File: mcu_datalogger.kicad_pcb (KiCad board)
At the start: 2 copper layers, 30.3 x 39.1 mm, 29 parts, among them J1 Conn_01x04_Pin, J2 Conn_01x04_Pin, J3 Conn_01x09_Pin, J4 Conn_02x03_Odd_Even, U1 24LC1025, U2 DS1337S_, U3 24LC1025, U4 ATMEGA328P-AU_SL044, Y1 32.768 KHz, Y2 16 MHz

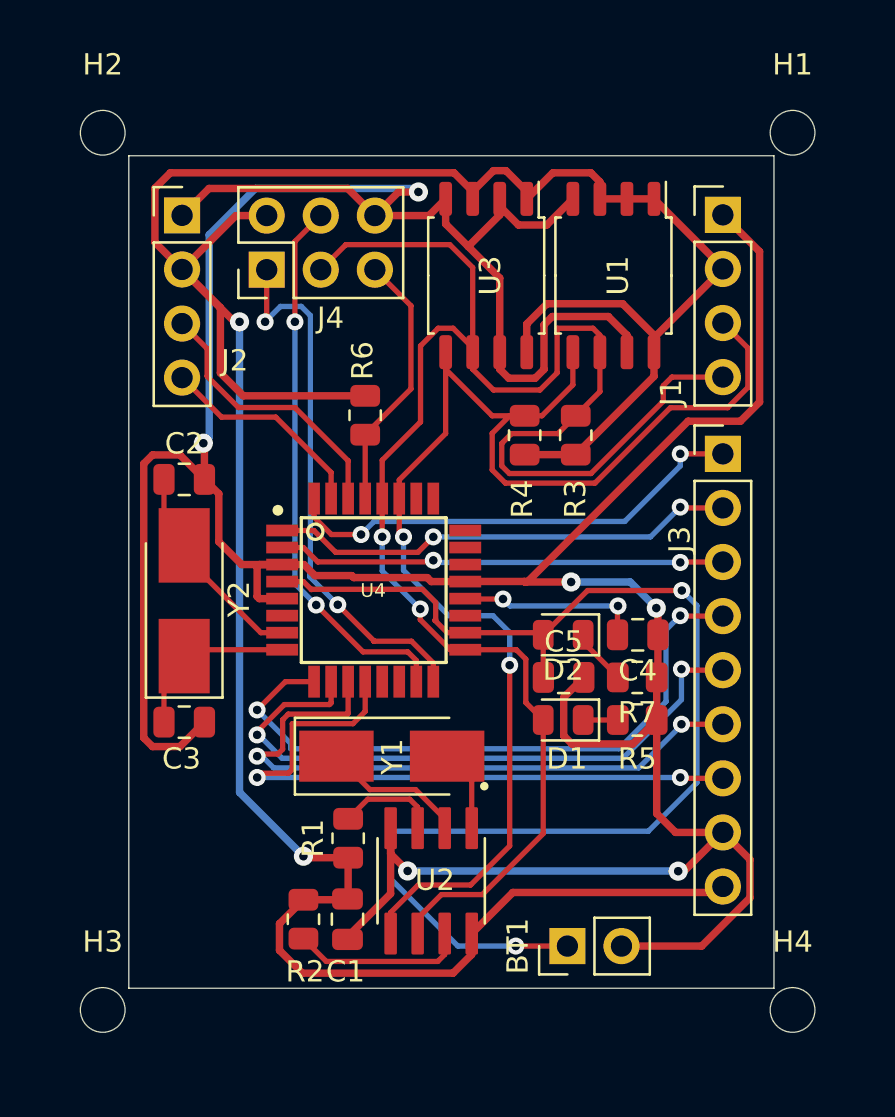
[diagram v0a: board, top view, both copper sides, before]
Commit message: PCB final
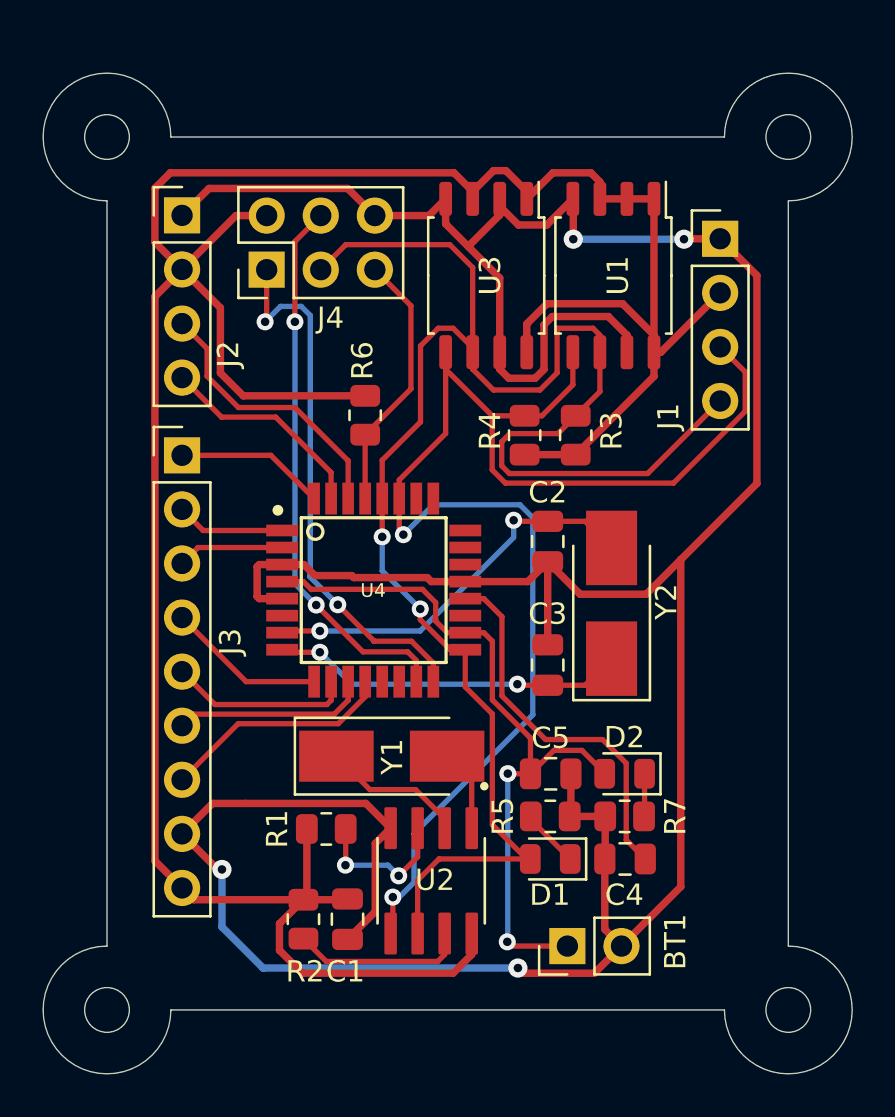
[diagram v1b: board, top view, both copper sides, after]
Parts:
- moved J3 25.4 mm to (146.5, 76.0)
- moved Y2 20.1 mm to (166.7, 82.9)
- moved C2 17.3 mm to (163.7, 80.0), turned to -90 degrees
- moved C3 17.3 mm to (163.7, 85.8), turned to 90 degrees
- moved C4 10.5 mm to (167.3, 94.9), turned to 0 degrees
- moved D2 7.14 mm to (167.3, 90.9)
- moved D1 6.56 mm to (163.8, 94.9)
- moved R7 6.55 mm to (167.3, 92.9), turned to 0 degrees
- moved R5 6.10 mm to (163.8, 92.9)
- moved C5 4.57 mm to (163.8, 90.9)
- moved J1 1.13 mm to (171.8, 65.8)
- moved R1 1.12 mm to (153.3, 93.5), turned to 0 degrees
- moved H1 0.28 mm to (175.0, 61.0)
- moved H2 0.28 mm to (143.0, 61.0)
- moved H3 0.20 mm to (143.0, 102.0)
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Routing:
- net GND: track 194.2 -> 166.9 mm, vias 6 -> 4
- net Net-(BT1-+): track 59.8 -> 34.9 mm
- net /D5: track 30.6 -> 7.45 mm, vias 2 -> 0
- net /D6: track 30.1 -> 8.60 mm, vias 2 -> 0
- net /D7: track 30.4 -> 9.17 mm, vias 2 -> 0
- net /D8: track 30.9 -> 10.9 mm, vias 2 -> 0
- net /D3: track 22.0 -> 5.11 mm, vias 2 -> 0
- net /D4: track 21.1 -> 5.01 mm, vias 2 -> 0
- net /D2: track 22.3 -> 7.04 mm, vias 2 -> 0
- net Net-(U4-AREF): track 8.68 -> 17.8 mm, vias 2 -> 0
- net Net-(U4-PB6): track 10.1 -> 18.7 mm, vias 0 -> 2
- net Net-(U4-PB7): track 8.22 -> 16.7 mm, vias 0 -> 2
- net /Vcc: track 139.6 -> 133.8 mm, vias 2 -> 0
- net Net-(U2-~{INTA}): track 4.79 -> 7.02 mm, vias 0 -> 2
- net /SDA: track 66.4 -> 68.3 mm
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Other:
- board size 30.3 x 39.1 mm -> 38 x 47 mm
